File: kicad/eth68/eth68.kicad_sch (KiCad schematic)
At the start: 75 parts, among them J14 Conn_02x10_Odd_Even, J201 Conn_01x02_Pin, J3 Conn_01x02_Pin, U201 PCM3168APAPR, U5 STM32H743ZIT6, Y1 SG-210STF

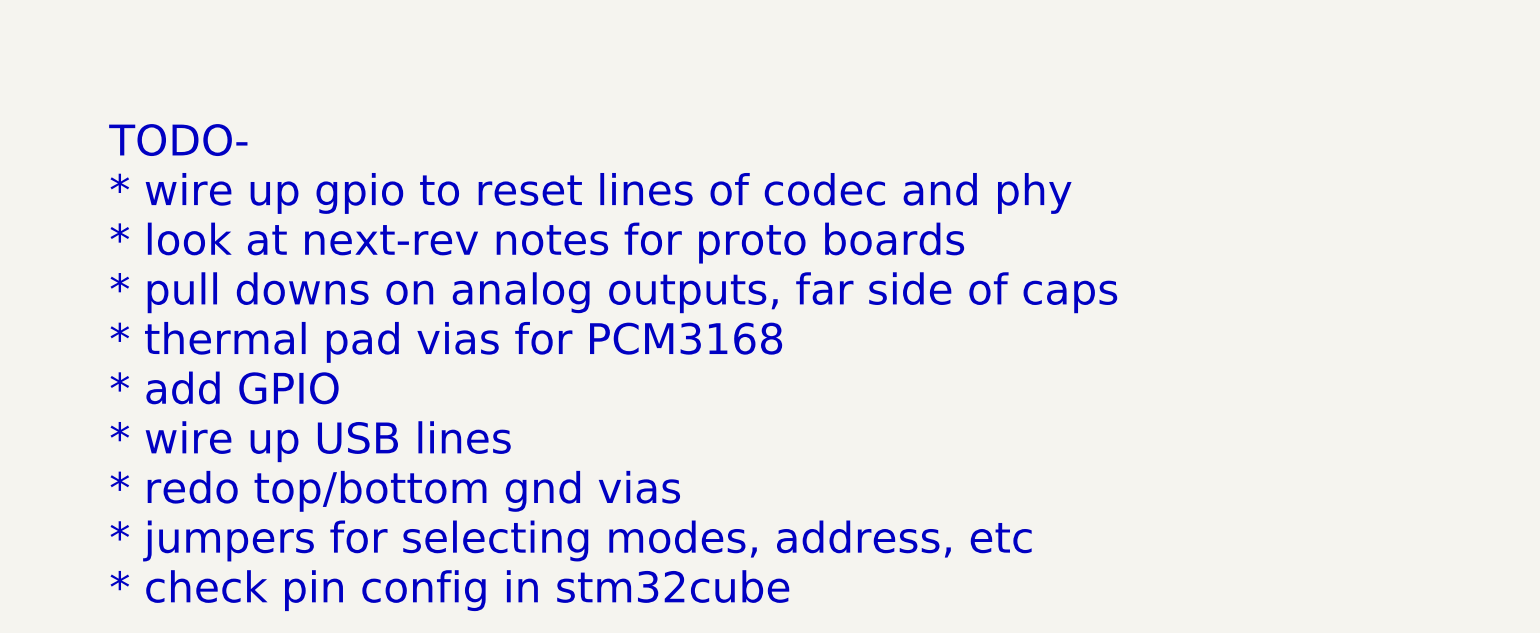
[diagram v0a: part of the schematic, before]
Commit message: WIP
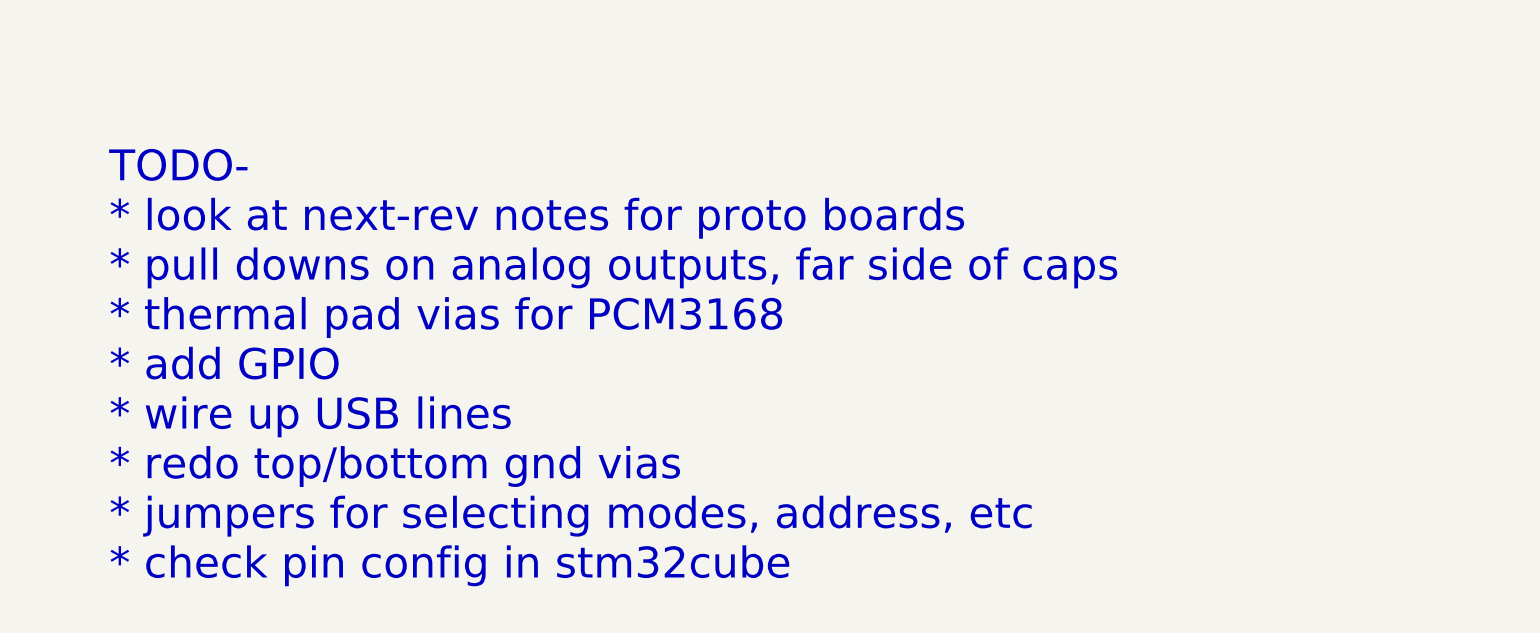
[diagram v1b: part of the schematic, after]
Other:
- note added: "TODO- * look at next-rev notes for proto boards * pull downs on analog outputs, far side of caps * thermal pad vias for PCM3168 * add GPIO * wire up USB lines * redo top/bottom gnd vias * jumpers for selecting modes, address, etc * check pin config in stm32cube"
- note removed: "TODO- * wire up gpio to reset lines of codec and phy * look at next-rev notes for proto boards * pull downs on analog outputs, far side of caps * thermal pad vias for PCM3168 * add GPIO * wire up USB lines * redo top/bottom gnd vias * jumpers for selecting modes, address, etc * check pin config in stm32cube"
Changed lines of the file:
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@@
 	(generator_version "9.0")
 	(paper "A1")
-	(text "TODO-\n* wire up gpio to reset lines of codec and phy\n* look at next-rev notes for proto boards\n* pull downs on analog outputs, far side of caps\n* thermal pad vias for PCM3168\n* add GPIO\n* wire up USB lines\n* redo top/bottom gnd vias\n* jumpers for selecting modes, address, etc\n* check pin config in stm32cube"
+	(text "TODO-\n* look at next-rev notes for proto boards\n* pull downs on analog outputs, far side of caps\n* thermal pad vias for PCM3168\n* add GPIO\n* wire up USB lines\n* redo top/bottom gnd vias\n* jumpers for selecting modes, address, etc\n* check pin config in stm32cube"
 		(exclude_from_sim no)
 		(at 853.694 477.266 0)
